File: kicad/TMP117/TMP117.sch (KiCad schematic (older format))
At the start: 7 parts, among them J1 Conn, J2 Conn, J3 Conn, J4 Conn

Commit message: изменено:      kicad/TMP117/TMP117-cache.lib 	изменено:      kicad/TMP117/TMP117.kicad_pcb 	изменено:      kicad/TMP117/TMP117.kicad_pcb-bak 	изменено:      kicad/TMP117/TMP117.sch 	изменено:      kicad/TMP117/TMP117.sch-bak
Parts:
- added C1: 0.1uF, Capacitor_SMD:C_0402_1005Metric, symbol Device:C
- D1: symbol My_Library:TMP117 -> TMP117-rescue:TMP117-My_Library
- J1, J2, J3, J4: symbol My_Library:Conn -> TMP117-rescue:Conn-My_Library
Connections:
- wire segments 15 -> 16
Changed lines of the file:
@@
 $EndDescr
 $Comp
-L My_Library:TMP117 D1
+L TMP117-rescue:TMP117-My_Library D1
 U 1 1 623AF833
 P 5450 2500
@@
 P 5450 3050
 F 0 "#PWR0101" H 5450 2800 50  0001 C CNN
-F 1 "GND" H 5455 2877 50  0000 C CNN
+F 1 "GND" H 5455 2877 50  0001 C CNN
 F 2 "" H 5450 3050 50  0001 C CNN
 F 3 "" H 5450 3050 50  0001 C CNN
@@
 $EndComp
 $Comp
-L My_Library:Conn J1
+L TMP117-rescue:Conn-My_Library J1
 U 1 1 623B0AA1
 P 4800 1850
@@
 $EndComp
 $Comp
-L My_Library:Conn J2
+L TMP117-rescue:Conn-My_Library J2
 U 1 1 623B0F07
 P 4800 2400
@@
 $EndComp
 $Comp
-L My_Library:Conn J3
+L TMP117-rescue:Conn-My_Library J3
 U 1 1 623B1137
 P 4800 2650
@@
 $EndComp
 $Comp
-L My_Library:Conn J4
+L TMP117-rescue:Conn-My_Library J4
 U 1 1 623B1419
 P 4800 3050
@@
 	5450 1850 5450 2150
 Connection ~ 5450 1850
+$Comp
+L Device:C C1
+U 1 1 6249AFED
+P 5900 2000
+F 0 "C1" H 6015 2046 50  0000 L CNN
+F 1 "0.1uF" H 6015 1955 50  0000 L CNN
+F 2 "Capacitor_SMD:C_0402_1005Metric" H 5938 1850 50  0001 C CNN
+F 3 "~" H 5900 2000 50  0001 C CNN
+	1    5900 2000
+	1    0    0    -1
+$EndComp
+Wire Wire Line
+	5450 1850 5900 1850
+$Comp
+L power:GND #PWR0103
+U 1 1 6249B84F
+P 5900 2150
+F 0 "#PWR0103" H 5900 1900 50  0001 C CNN
+F 1 "GND" H 5905 1977 50  0001 C CNN
+F 2 "" H 5900 2150 50  0001 C CNN
+F 3 "" H 5900 2150 50  0001 C CNN
+	1    5900 2150
+	1    0    0    -1
+$EndComp
 $EndSCHEMATC

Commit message: изменено:      kicad/TMP117/TMP117-cache.lib 	изменено:      kicad/TMP117/TMP117.kicad_pcb 	изменено:      kicad/TMP117/TMP117.kicad_pcb-bak 	изменено:      kicad/TMP117/TMP117.sch 	изменено:      kicad/TMP117/TMP117.sch-bak
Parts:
- D1: symbol TMP117-rescue:TMP117-My_Library -> TMP117-rescue:TMP117-My_Library-TMP117-rescue
- J1, J2, J3, J4: symbol TMP117-rescue:Conn-My_Library -> TMP117-rescue:Conn-My_Library-TMP117-rescue
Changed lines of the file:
@@
 $EndDescr
 $Comp
-L TMP117-rescue:TMP117-My_Library D1
+L TMP117-rescue:TMP117-My_Library-TMP117-rescue D1
 U 1 1 623AF833
 P 5450 2500
@@
 $EndComp
 $Comp
-L TMP117-rescue:Conn-My_Library J1
+L TMP117-rescue:Conn-My_Library-TMP117-rescue J1
 U 1 1 623B0AA1
 P 4800 1850
@@
 $EndComp
 $Comp
-L TMP117-rescue:Conn-My_Library J2
+L TMP117-rescue:Conn-My_Library-TMP117-rescue J2
 U 1 1 623B0F07
 P 4800 2400
@@
 $EndComp
 $Comp
-L TMP117-rescue:Conn-My_Library J3
+L TMP117-rescue:Conn-My_Library-TMP117-rescue J3
 U 1 1 623B1137
 P 4800 2650
@@
 $EndComp
 $Comp
-L TMP117-rescue:Conn-My_Library J4
+L TMP117-rescue:Conn-My_Library-TMP117-rescue J4
 U 1 1 623B1419
 P 4800 3050

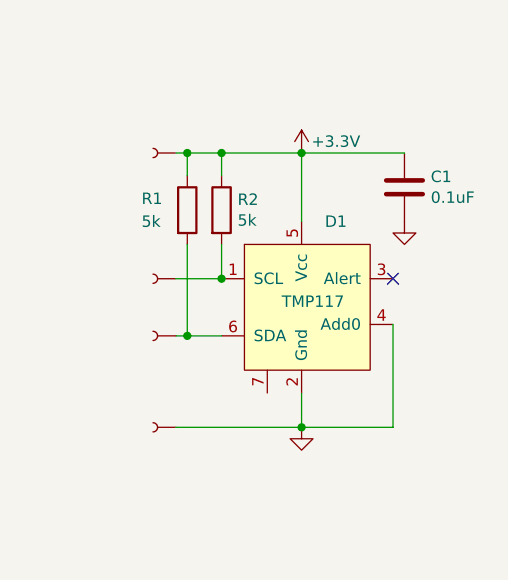
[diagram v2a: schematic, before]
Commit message: новый файл:    Documents/TMP117.png 	изменено:      kicad/TMP117/TMP117-cache.lib 	изменено:      kicad/TMP117/TMP117.sch 	изменено:      kicad/TMP117/TMP117.sch-bak
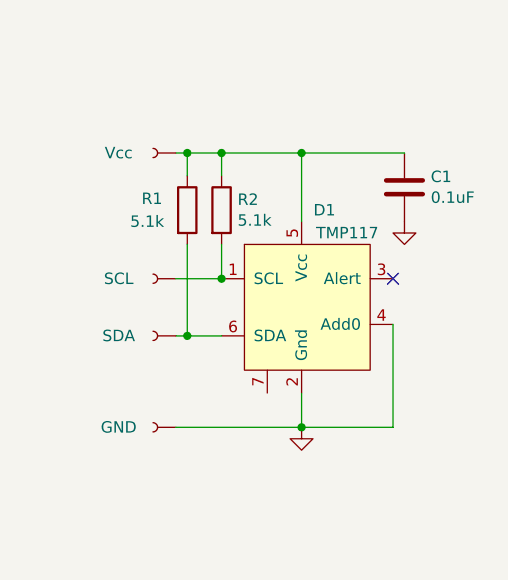
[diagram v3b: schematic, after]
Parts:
- J1: value Conn -> Vcc
- J2: value Conn -> SCL
- J3: value Conn -> SDA
- J4: value Conn -> GND
- R1, R2: value 5k -> 5.1k
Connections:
- net +3V3: no longer names the net of C1.1, D1.5 (Vcc), J1.1, R1.1, R2.1
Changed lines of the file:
@@
 U 1 1 623AF833
 P 5450 2500
-F 0 "D1" H 5600 2850 50  0000 C CNN
-F 1 "TMP117" H 5500 2500 50  0000 C CNN
+F 0 "D1" H 5550 2900 50  0000 C CNN
+F 1 "TMP117" H 5650 2800 50  0000 C CNN
 F 2 "My-library:TMP117" H 5250 2300 50  0001 C CNN
 F 3 "" H 5250 2300 50  0001 C CNN
@@
 NoConn ~ 5850 2400
 $Comp
-L power:+3.3V #PWR0102
-U 1 1 623B0130
-P 5450 1850
-F 0 "#PWR0102" H 5450 1700 50  0001 C CNN
-F 1 "+3.3V" H 5600 1900 50  0000 C CNN
-F 2 "" H 5450 1850 50  0001 C CNN
-F 3 "" H 5450 1850 50  0001 C CNN
-	1    5450 1850
-	1    0    0    -1
-$EndComp
-$Comp
 L TMP117-rescue:Conn-My_Library-TMP117-rescue J1
 U 1 1 623B0AA1
 P 4800 1850
 F 0 "J1" H 4742 1665 50  0001 C CNN
-F 1 "Conn" H 4742 1756 50  0001 C CNN
+F 1 "Vcc" H 4950 1850 50  0000 C CNN
 F 2 "My-library:SMD-CONN" H 4850 1700 50  0001 C CNN
 F 3 "~" H 4800 1850 50  0001 C CNN
@@
 P 4800 2400
 F 0 "J2" H 4742 2215 50  0001 C CNN
-F 1 "Conn" H 4742 2306 50  0001 C CNN
+F 1 "SCL" H 4950 2400 50  0000 C CNN
 F 2 "My-library:SMD-CONN" H 4850 2250 50  0001 C CNN
 F 3 "~" H 4800 2400 50  0001 C CNN
@@
 P 4800 2650
 F 0 "J3" H 4742 2465 50  0001 C CNN
-F 1 "Conn" H 4742 2556 50  0001 C CNN
+F 1 "SDA" H 4950 2650 50  0000 C CNN
 F 2 "My-library:SMD-CONN" H 4850 2500 50  0001 C CNN
 F 3 "~" H 4800 2650 50  0001 C CNN
@@
 P 4800 3050
 F 0 "J4" H 4742 2865 50  0001 C CNN
-F 1 "Conn" H 4742 2956 50  0001 C CNN
+F 1 "GND" H 4950 3050 50  0000 C CNN
 F 2 "My-library:SMD-CONN" H 4850 2900 50  0001 C CNN
 F 3 "~" H 4800 3050 50  0001 C CNN
@@
 P 4950 2100
 F 0 "R1" H 4750 2150 50  0000 L CNN
-F 1 "5k" H 4750 2050 50  0000 L CNN
+F 1 "5.1k" H 4700 2050 50  0000 L CNN
 F 2 "Resistor_SMD:R_0402_1005Metric" V 4880 2100 50  0001 C CNN
 F 3 "~" H 4950 2100 50  0001 C CNN
@@
 P 5100 2100
 F 0 "R2" H 5170 2146 50  0000 L CNN
-F 1 "5k" H 5170 2055 50  0000 L CNN
+F 1 "5.1k" H 5170 2055 50  0000 L CNN
 F 2 "Resistor_SMD:R_0402_1005Metric" V 5030 2100 50  0001 C CNN
 F 3 "~" H 5100 2100 50  0001 C CNN

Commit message: изменено:      kicad/TMP117/TMP117-cache.lib 	изменено:      kicad/TMP117/TMP117.kicad_pcb 	изменено:      kicad/TMP117/TMP117.kicad_pcb-bak 	изменено:      kicad/TMP117/TMP117.sch 	изменено:      kicad/TMP117/TMP117.sch-bak
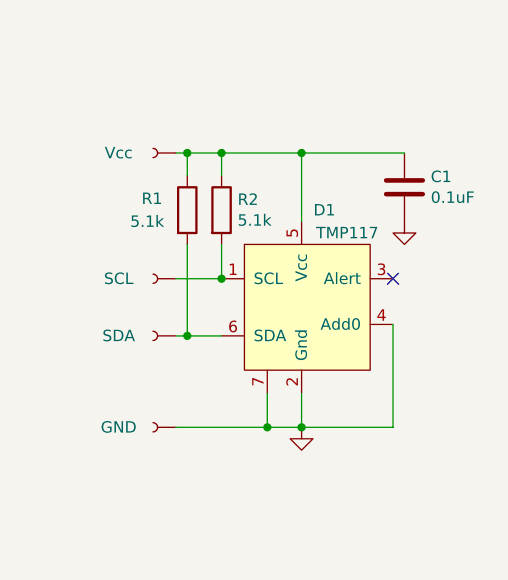
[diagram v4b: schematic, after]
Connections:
- net GND: now also D1.7
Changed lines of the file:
@@
 $EndComp
-Wire Wire Line
-	4900 3050 5450 3050
 Wire Wire Line
 	4900 2650 4950 2650
@@
 	1    0    0    -1
 $EndComp
+Wire Wire Line
+	4900 3050 5300 3050
+Wire Wire Line
+	5300 2900 5300 3050
+Connection ~ 5300 3050
+Wire Wire Line
+	5300 3050 5450 3050
 $EndSCHEMATC

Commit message: изменено:      kicad/Anemometr/Anemometr.sch 	изменено:      kicad/Anemometr/Anemometr.sch-bak 	изменено:      kicad/TMP117/TMP117-cache.lib 	изменено:      kicad/TMP117/TMP117.sch 	изменено:      kicad/TMP117/TMP117.sch-bak 	изменено:      stm32cubeide/Anemometer/Core/Inc/main.h 	новый файл:    stm32cubeide/Anemometer/Core/Inc/tmp117.h 	изменено:      stm32cubeide/Anemometer/Core/Src/main.c 	новый файл:    stm32cubeide/Anemometer/Core/Src/tmp117.c 	изменено:      stm32cubeide/Anemometer/Release/Anemometer.bin 	изменено:      stm32cubeide/Anemometer/Release/Anemometer.elf 	изменено:      stm32cubeide/Anemometer/Release/Anemometer.list 	изменено:      stm32cubeide/Anemometer/Release/Anemometer.map 	изменено:      stm32cubeide/Anemometer/Release/Core/Src/main.d 	изменено:      stm32cubeide/Anemometer/Release/Core/Src/main.o 	изменено:      stm32cubeide/Anemometer/Release/Core/Src/main.su 	изменено:      stm32cubeide/Anemometer/Release/Core/Src/stm32f1xx_hal_msp.d 	изменено:      stm32cubeide/Anemometer/Release/Core/Src/stm32f1xx_hal_msp.o 	изменено:      stm32cubeide/Anemometer/Release/Core/Src/stm32f1xx_it.d 	изменено:      stm32cubeide/Anemometer/Release/Core/Src/stm32f1xx_it.o 	изменено:      stm32cubeide/Anemometer/Release/Core/Src/subdir.mk 	изменено:      stm32cubeide/Anemometer/Release/objects.list
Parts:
- D1: symbol TMP117-rescue:TMP117-My_Library-TMP117-rescue -> TMP117-rescue:TMP117-My_Library-TMP117-rescue-TMP117-rescue
- J1, J2, J3, J4: symbol TMP117-rescue:Conn-My_Library-TMP117-rescue -> TMP117-rescue:Conn-My_Library-TMP117-rescue-TMP117-rescue
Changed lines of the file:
@@
 $EndDescr
 $Comp
-L TMP117-rescue:TMP117-My_Library-TMP117-rescue D1
+L TMP117-rescue:TMP117-My_Library-TMP117-rescue-TMP117-rescue D1
 U 1 1 623AF833
 P 5450 2500
@@
 NoConn ~ 5850 2400
 $Comp
-L TMP117-rescue:Conn-My_Library-TMP117-rescue J1
+L TMP117-rescue:Conn-My_Library-TMP117-rescue-TMP117-rescue J1
 U 1 1 623B0AA1
 P 4800 1850
@@
 $EndComp
 $Comp
-L TMP117-rescue:Conn-My_Library-TMP117-rescue J2
+L TMP117-rescue:Conn-My_Library-TMP117-rescue-TMP117-rescue J2
 U 1 1 623B0F07
 P 4800 2400
@@
 $EndComp
 $Comp
-L TMP117-rescue:Conn-My_Library-TMP117-rescue J3
+L TMP117-rescue:Conn-My_Library-TMP117-rescue-TMP117-rescue J3
 U 1 1 623B1137
 P 4800 2650
@@
 $EndComp
 $Comp
-L TMP117-rescue:Conn-My_Library-TMP117-rescue J4
+L TMP117-rescue:Conn-My_Library-TMP117-rescue-TMP117-rescue J4
 U 1 1 623B1419
 P 4800 3050
